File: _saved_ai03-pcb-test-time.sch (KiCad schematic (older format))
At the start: 24 parts, among them SW1 SW_Push, U1 ATmega32U4-AU, Y1 16MHz

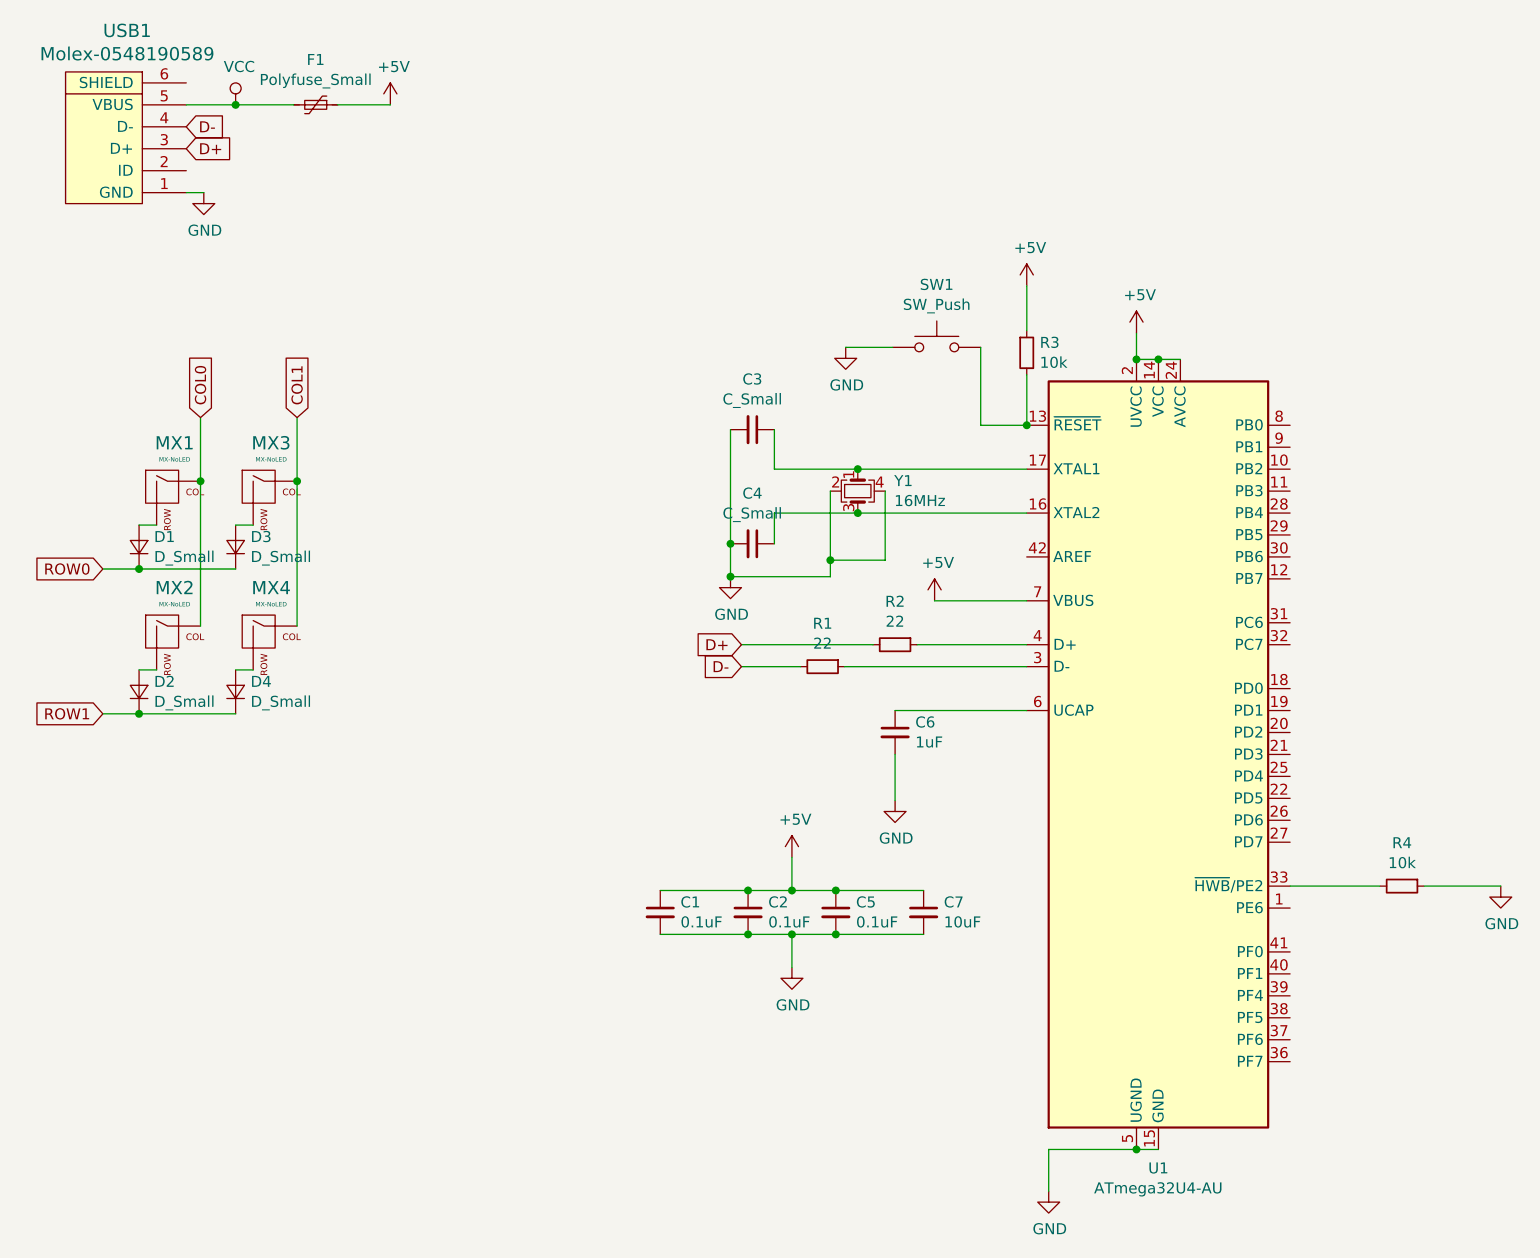
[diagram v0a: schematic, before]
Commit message: Revert "Schematic completed"
This reverts commit 1cac4397530574a4662a2747fb7876ea94054bb6.
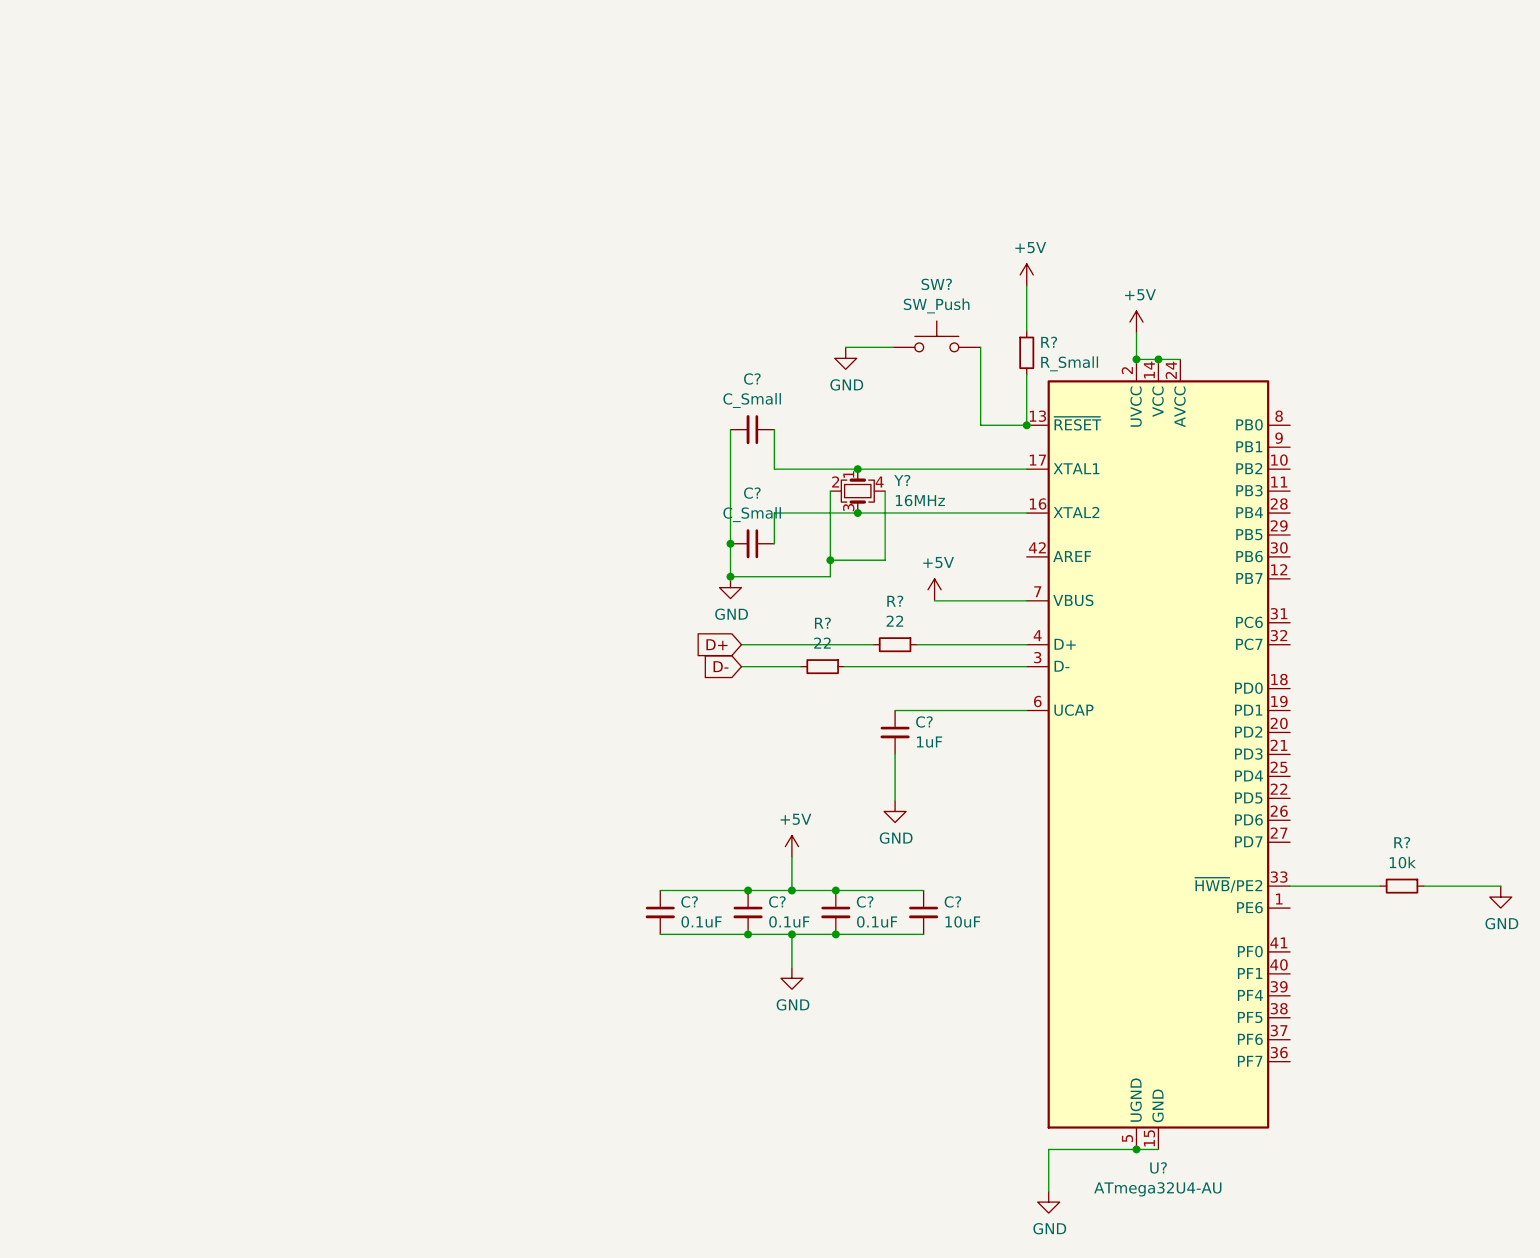
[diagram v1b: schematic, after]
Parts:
- removed D1, D2, D3, D4: D_Small, Diode_SMD:D_SOD-123, symbol Device:D_Small
- removed F1: Polyfuse_Small, Fuse:Fuse_1206_3216Metric, symbol Device:Polyfuse_Small
- removed MX1, MX2, MX3, MX4: MX-NoLED, MX_Alps_Hybrid:MX-1U-NoLED, symbol MX_Alps_Hybrid:MX-NoLED
- removed USB1: Molex-0548190589, random-keyboard-parts:Molex-0548190589, symbol random-keyboard-parts:Molex-0548190589
- C?: renamed from C1; footprint Capacitor_SMD:C_0805_2012Metric -> (none)
- C?: renamed from C6; footprint Capacitor_SMD:C_0805_2012Metric -> (none)
- C?: renamed from C2; footprint Capacitor_SMD:C_0805_2012Metric -> (none)
- C?: renamed from C5; footprint Capacitor_SMD:C_0805_2012Metric -> (none)
- C?: renamed from C7; footprint Capacitor_SMD:C_0805_2012Metric -> (none)
- C?: renamed from C3; footprint Capacitor_SMD:C_0805_2012Metric -> (none)
- C?: renamed from C4; footprint Capacitor_SMD:C_0805_2012Metric -> (none)
- R?: renamed from R4; footprint Resistor_SMD:R_0805_2012Metric -> (none)
- R?: renamed from R2; footprint Resistor_SMD:R_0805_2012Metric -> (none)
- R?: renamed from R1; footprint Resistor_SMD:R_0805_2012Metric -> (none)
- R?: renamed from R3; value 10k -> R_Small; footprint Resistor_SMD:R_0805_2012Metric -> (none)
- SW?: renamed from SW1; footprint random-keyboard-parts:SKQG-1155865 -> (none)
- Y?: renamed from Y1; footprint Crystal:Crystal_SMD_3225-4Pin_3.2x2.5mm -> (none)
- renumbered U1 to U?

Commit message: Schematic completed
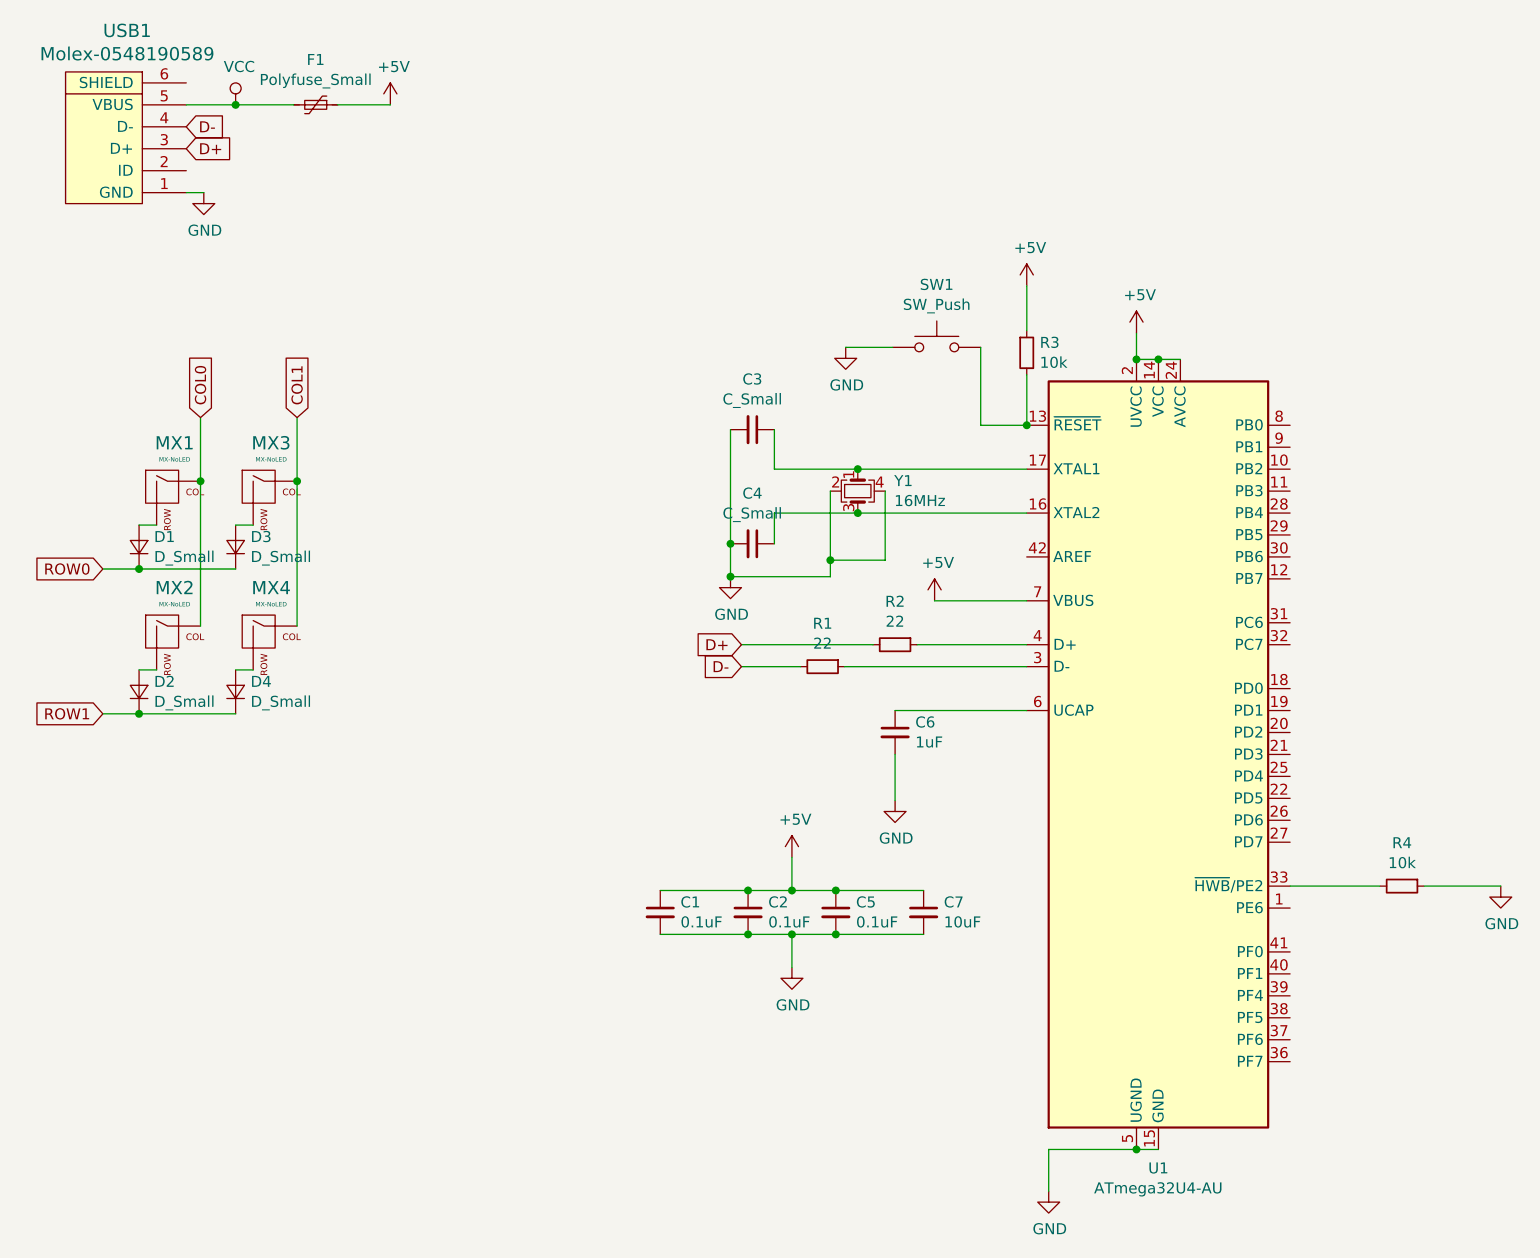
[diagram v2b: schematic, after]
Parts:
- added D1, D2, D3, D4: D_Small, Diode_SMD:D_SOD-123, symbol Device:D_Small
- added F1: Polyfuse_Small, Fuse:Fuse_1206_3216Metric, symbol Device:Polyfuse_Small
- added MX1, MX2, MX3, MX4: MX-NoLED, MX_Alps_Hybrid:MX-1U-NoLED, symbol MX_Alps_Hybrid:MX-NoLED
- added USB1: Molex-0548190589, random-keyboard-parts:Molex-0548190589, symbol random-keyboard-parts:Molex-0548190589
- C1, C2, C3, C4, C5, C6, C7: renamed from C?; footprint (none) -> Capacitor_SMD:C_0805_2012Metric
- R1, R2, R4: renamed from R?; footprint (none) -> Resistor_SMD:R_0805_2012Metric
- R3: renamed from R?; value R_Small -> 10k; footprint (none) -> Resistor_SMD:R_0805_2012Metric
- SW1: renamed from SW?; footprint (none) -> random-keyboard-parts:SKQG-1155865
- Y1: renamed from Y?; footprint (none) -> Crystal:Crystal_SMD_3225-4Pin_3.2x2.5mm
- gave numbers to parts that had none: 1
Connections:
- net +5V: now also F1.1
- net D+: now also USB1.3 (D+)
- net D-: now also USB1.4 (D-)
- net GND: now also USB1.1 (GND)
- new net: D1.2 (A), MX1.2 (ROW)
- new net: D3.2 (A), MX3.2 (ROW)
- new net: D2.2 (A), MX2.2 (ROW)
- new net: D4.2 (A), MX4.2 (ROW)
- new net COL0: MX1.1 (COL), MX2.1 (COL)
- new net COL1: MX3.1 (COL), MX4.1 (COL)
- new net ROW0: D1.1 (K), D3.1 (K)
- new net ROW1: D2.1 (K), D4.1 (K)
- new net VCC: F1.2, USB1.5 (VBUS)
